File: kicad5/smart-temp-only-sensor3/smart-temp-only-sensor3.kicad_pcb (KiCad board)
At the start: 2 copper layers, 2 parts, among them J1 USB_B_Mini, J2 Conn_01x04_Female

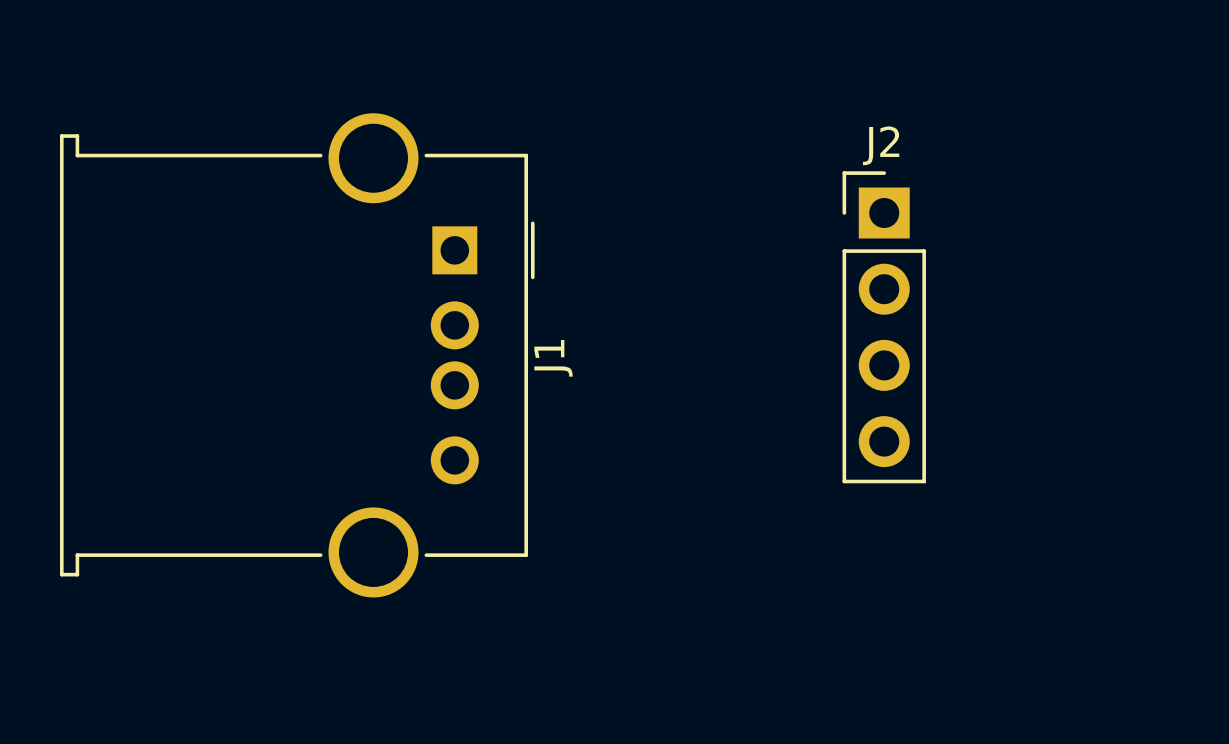
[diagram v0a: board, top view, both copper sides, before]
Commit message: noid: autoroute final beta
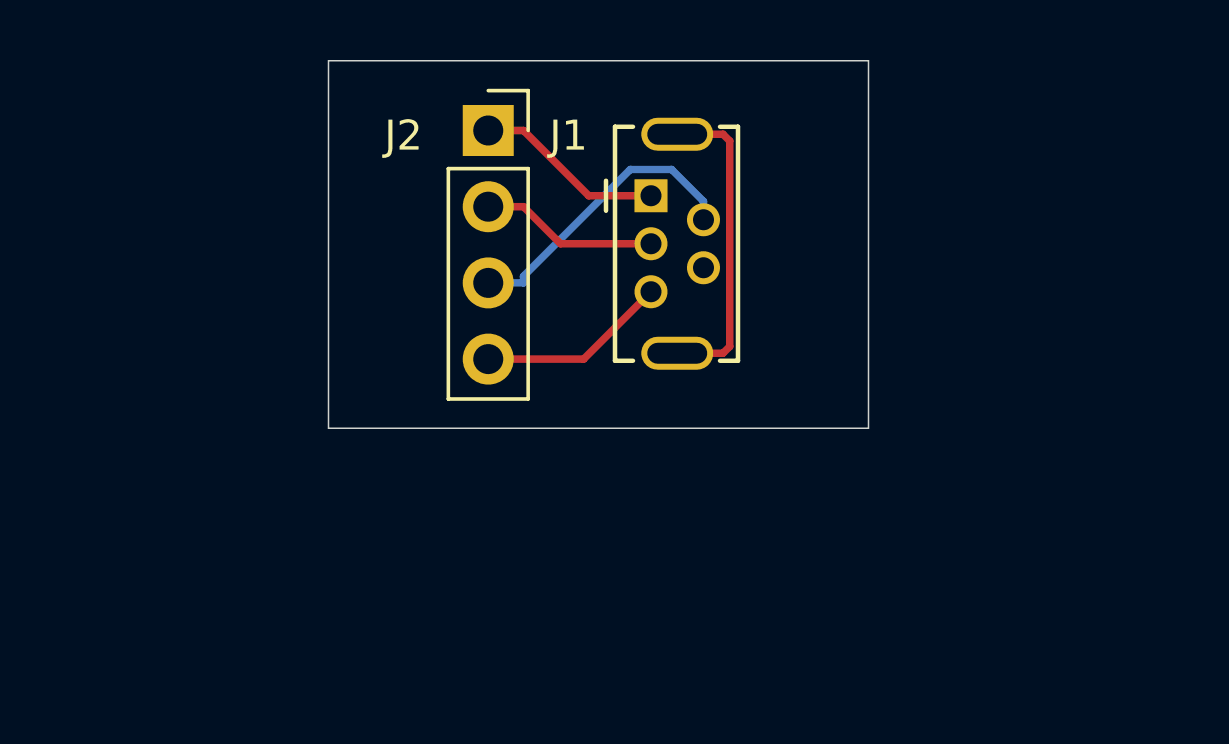
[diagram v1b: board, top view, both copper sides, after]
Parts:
- J1: footprint Connector_USB:USB_A_Molex_67643_Horizontal -> Connector_USB:USB_Mini-B_Tensility_54-00023_Vertical
- J2: footprint Connector_PinHeader_2.54mm:PinHeader_1x04_P2.54mm_Vertical -> Connector_PinSocket_2.54mm:PinSocket_1x04_P2.54mm_Vertical
- moved J2 13.5 mm to (76.8, 60.3)
- moved J1 6.79 mm to (82.2, 62.5)
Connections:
- J1 pad 1: Net-(J1-Pad1) -> +3V3
- J1 pad 5: Net-(J1-Pad5) -> GND1
- J2 pad 1: Net-(J2-Pad1) -> +3V3
- J2 pad 2: Net-(J2-Pad2) -> Net-(J1-Pad3)
- J2 pad 3: Net-(J2-Pad3) -> Net-(J1-Pad2)
- J2 pad 4: Net-(J2-Pad4) -> GND1
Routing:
- net Net-(J1-Pad6): track 0.00 -> 10.5 mm
- net Net-(J1-Pad2): track 0.00 -> 9.92 mm
- net GND1: track 0.00 -> 6.35 mm
- net +3V3: track 0.00 -> 6.33 mm
- net Net-(J1-Pad3): track 0.00 -> 5.94 mm
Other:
- board outline added: 18 x 12.2 mm

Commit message: smart-temp-only-sensor3
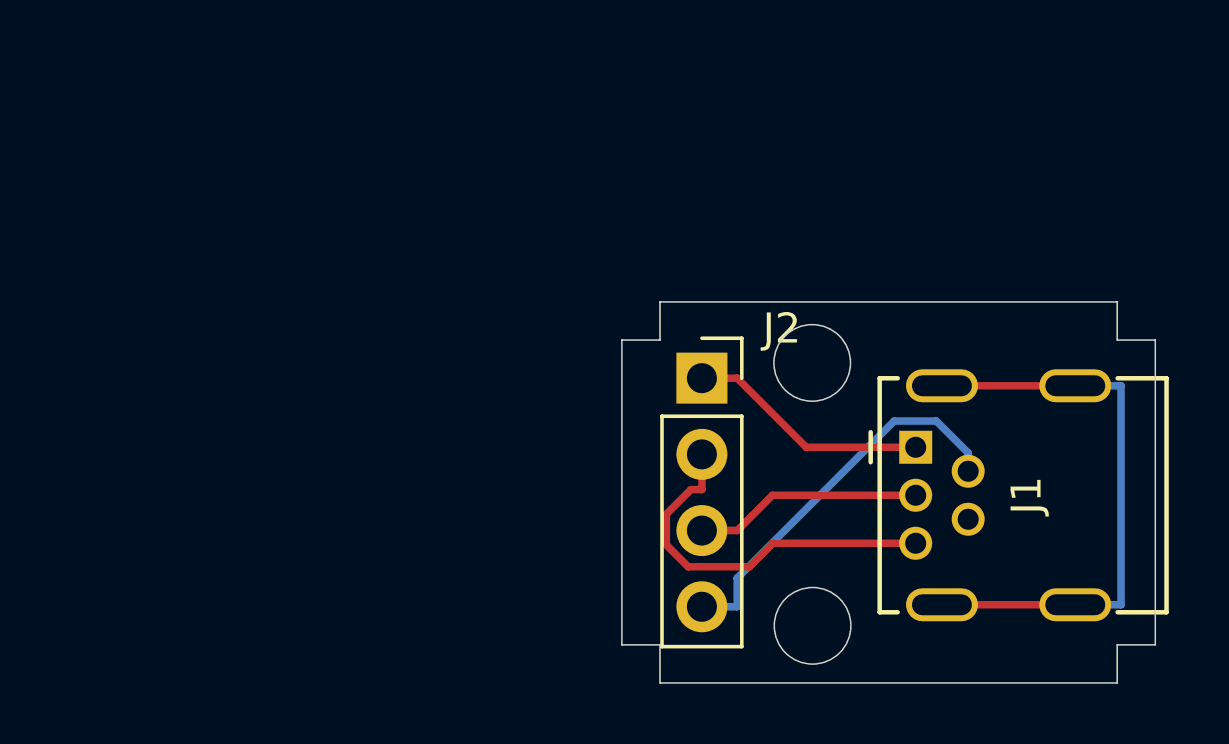
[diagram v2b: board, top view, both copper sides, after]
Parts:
- J1: footprint Connector_USB:USB_Mini-B_Tensility_54-00023_Vertical -> kicad3_footprint:USB_Mini-B_econ_connect_vertical
- J2: value Conn_01x04_Female -> Conn_Female
- moved J1 12.2 mm to (91.1, 70.9)
- moved J2 10.9 mm to (83.9, 68.6)
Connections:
- J1 pad 2: Net-(J1-Pad2) -> /SDA_GPIO_0
- J1 pad 3: Net-(J1-Pad3) -> /SDL_GPIO_2
- J2 pad 2: Net-(J1-Pad3) -> GND1
- J2 pad 3: Net-(J1-Pad2) -> /SDL_GPIO_2
- J2 pad 4: GND1 -> /SDA_GPIO_0
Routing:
- net /SDA_GPIO_0: track 0.00 -> 13.1 mm
- net Net-(J1-Pad2): track 9.92 -> 0.00 mm
- net Net-(J1-Pad6): track 10.5 -> 19.2 mm
- net /SDL_GPIO_2: track 0.00 -> 7.61 mm
- net GND1: track 6.35 -> 12.7 mm
- net Net-(J1-Pad3): track 5.94 -> 0.00 mm
- net +3V3: track 6.33 -> 8.08 mm
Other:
- board size 18 x 12.2 mm -> 17.8 x 12.7 mm
